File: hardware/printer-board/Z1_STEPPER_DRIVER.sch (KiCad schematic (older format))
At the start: 9 parts, among them J10 Z1, J9 MS_SELECT, U6 A4988_MODULE

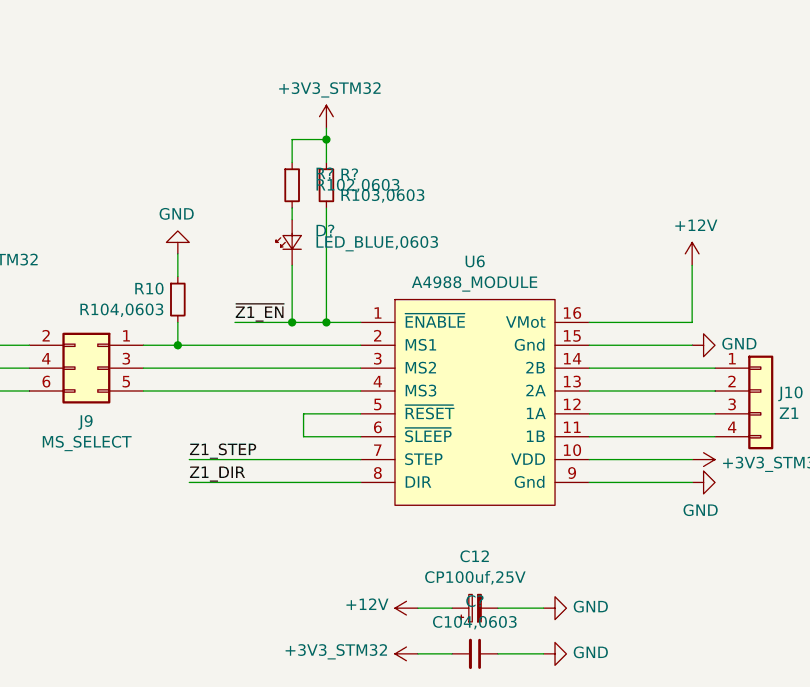
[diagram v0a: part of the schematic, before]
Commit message: update annotations,
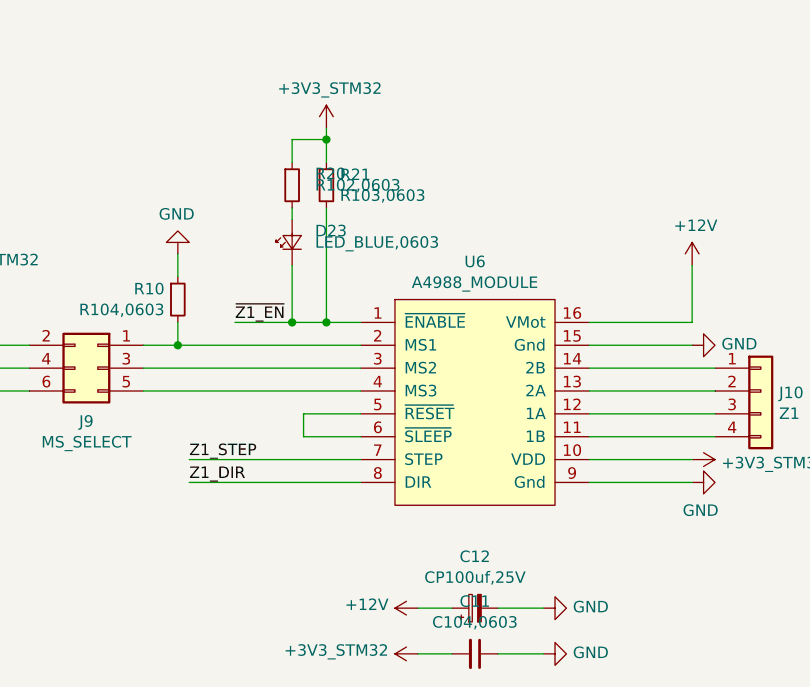
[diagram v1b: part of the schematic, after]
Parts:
- gave numbers to parts that had none: 4
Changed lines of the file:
@@
 $EndBitmap
 $Comp
-L taobao-components:+3V3_STM32 #PWR?
+L taobao-components:+3V3_STM32 #PWR019
 U 1 1 5CC40A85
 P 3500 2700
-F 0 "#PWR?" H 3500 2550 50  0001 C CNN
+F 0 "#PWR019" H 3500 2550 50  0001 C CNN
 F 1 "+3V3_STM32" H 3515 2873 50  0000 C CNN
 F 2 "" H 3500 2700 50  0001 C CNN
@@
 $EndComp
 $Comp
-L taobao-components:+3V3_STM32 #PWR?
+L taobao-components:+3V3_STM32 #PWR021
 U 1 1 5CC40A9C
 P 5400 4250
-F 0 "#PWR?" H 5400 4100 50  0001 C CNN
+F 0 "#PWR021" H 5400 4100 50  0001 C CNN
 F 1 "+3V3_STM32" V 5415 4378 50  0000 L CNN
 F 2 "" H 5400 4250 50  0001 C CNN
@@
 $EndComp
 $Comp
-L taobao-components:+3V3_STM32 #PWR?
+L taobao-components:+3V3_STM32 #PWR020
 U 1 1 5CC40AC5
 P 6600 3400
-F 0 "#PWR?" H 6600 3250 50  0001 C CNN
+F 0 "#PWR020" H 6600 3250 50  0001 C CNN
 F 1 "+3V3_STM32" V 6615 3528 50  0000 L CNN
 F 2 "" H 6600 3400 50  0001 C CNN
@@
 $EndComp
 $Comp
-L taobao-c:C104,0603 C?
+L taobao-c:C104,0603 C11
 U 1 1 5CC40BBB
 P 5650 4250
-F 0 "C?" V 5421 4250 50  0000 C CNN
+F 0 "C11" V 5421 4250 50  0000 C CNN
 F 1 "C104,0603" V 5512 4250 50  0000 C CNN
 F 2 "Capacitor_SMD:C_0603_1608Metric_Pad1.05x0.95mm_HandSolder" H 5650 4250 50  0001 C CNN
@@
 AR Path="/5CC0A4B9/5CC5991B" Ref="R?"  Part="1"
 AR Path="/5CC0A53C/5CC5991B" Ref="R?"  Part="1"
-AR Path="/5CC0A8C5/5CC5991B" Ref="R?"  Part="1"
+AR Path="/5CC0A8C5/5CC5991B" Ref="R21"  Part="1"
 AR Path="/5CC0A8CA/5CC5991B" Ref="R?"  Part="1"
 AR Path="/5CC0A8CF/5CC5991B" Ref="R?"  Part="1"
 AR Path="/5CC0AEC9/5CC5991B" Ref="R?"  Part="1"
-F 0 "R?" H 5059 2246 50  0000 L CNN
+F 0 "R21" H 5059 2246 50  0000 L CNN
 F 1 "R103,0603" H 5059 2155 50  0000 L CNN
 F 2 "Resistor_SMD:R_0603_1608Metric_Pad1.05x0.95mm_HandSolder" H 5000 2200 50  0001 C CNN
@@
 P 5000 1950
 AR Path="/5CC0AEC9/5CC59923" Ref="#PWR?"  Part="1"
-AR Path="/5CC0A8C5/5CC59923" Ref="#PWR?"  Part="1"
-F 0 "#PWR?" H 5000 1800 50  0001 C CNN
+AR Path="/5CC0A8C5/5CC59923" Ref="#PWR018"  Part="1"
+F 0 "#PWR018" H 5000 1800 50  0001 C CNN
 F 1 "+3V3_STM32" H 5015 2123 50  0000 C CNN
 F 2 "" H 5000 1950 50  0001 C CNN
@@
 AR Path="/5CC15C35/5CC59929" Ref="R?"  Part="1"
 AR Path="/5CC0AEC9/5CC59929" Ref="R?"  Part="1"
-AR Path="/5CC0A8C5/5CC59929" Ref="R?"  Part="1"
-F 0 "R?" H 4950 2250 50  0000 L CNN
+AR Path="/5CC0A8C5/5CC59929" Ref="R20"  Part="1"
+F 0 "R20" H 4950 2250 50  0000 L CNN
 F 1 "R102,0603" H 4950 2200 50  0000 L CNN
 F 2 "Resistor_SMD:R_0603_1608Metric_Pad1.05x0.95mm_HandSolder" H 4850 2200 50  0001 C CNN
@@
 AR Path="/5CC15C35/5CC59930" Ref="D?"  Part="1"
 AR Path="/5CC0AEC9/5CC59930" Ref="D?"  Part="1"
-AR Path="/5CC0A8C5/5CC59930" Ref="D?"  Part="1"
-F 0 "D?" V 4900 2350 50  0000 R CNN
+AR Path="/5CC0A8C5/5CC59930" Ref="D23"  Part="1"
+F 0 "D23" V 4900 2350 50  0000 R CNN
 F 1 "LED_BLUE,0603" V 4850 2350 50  0000 R CNN
 F 2 "LED_SMD:LED_0603_1608Metric_Pad1.05x0.95mm_HandSolder" V 4850 2450 50  0001 C CNN

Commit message: update,
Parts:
- J10: footprint Connector_PinHeader_2.54mm:PinHeader_1x04_P2.54mm_Vertical -> footprint-lib:b4b-ph-kl,stepper_terminal
- U6: footprint Module:Pololu_Breakout-16_15.2x20.3mm -> footprint-lib:Pololu_Breakout-16_15.2x20.3mm
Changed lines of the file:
@@
 F 0 "U6" H 5650 3765 50  0000 C CNN
 F 1 "A4988_MODULE" H 5650 3674 50  0000 C CNN
-F 2 "Module:Pololu_Breakout-16_15.2x20.3mm" H 5650 3200 50  0001 C CNN
+F 2 "footprint-lib:Pololu_Breakout-16_15.2x20.3mm" H 5650 3200 50  0001 C CNN
 F 3 "" H 5650 3200 50  0001 C CNN
 	1    5650 3150
@@
 F 0 "J10" H 6980 3092 50  0000 L CNN
 F 1 "Z1" H 6980 3001 50  0000 L CNN
-F 2 "Connector_PinHeader_2.54mm:PinHeader_1x04_P2.54mm_Vertical" H 6900 3100 50  0001 C CNN
+F 2 "footprint-lib:b4b-ph-kl,stepper_terminal" H 6900 3100 50  0001 C CNN
 F 3 "~" H 6900 3100 50  0001 C CNN
 	1    6900 3100
